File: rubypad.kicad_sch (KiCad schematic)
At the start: 32 parts, among them J1 HRO-TYPE-C, SW1 SW_Push, SW2 RotaryEncoder_Switch, U1 ATmega32U4-A, Y1 16MHz

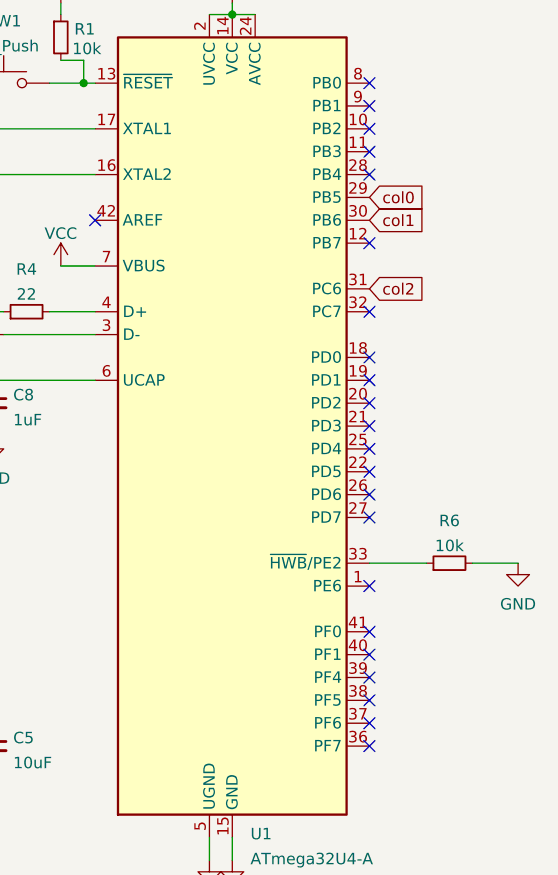
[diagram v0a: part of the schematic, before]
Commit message: changes and complete
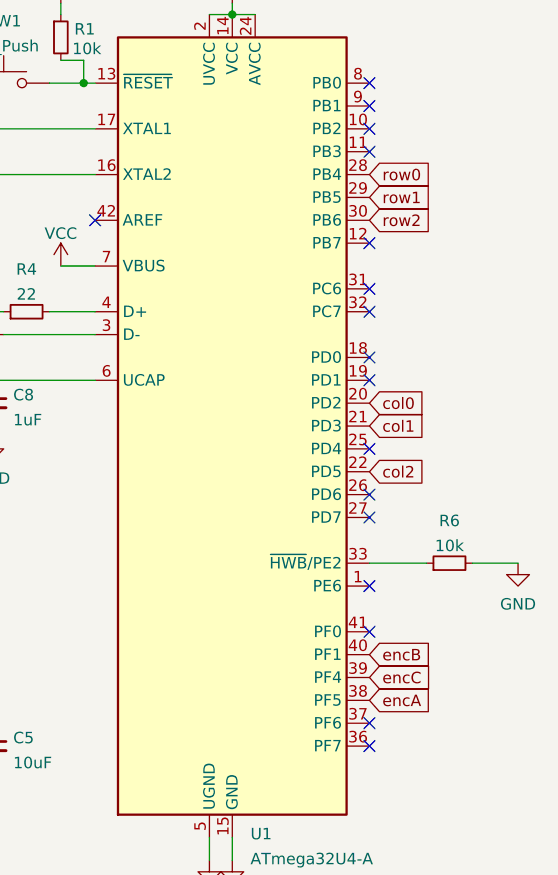
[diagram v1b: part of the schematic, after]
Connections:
- net col0: now also U1.20 (PD2); no longer U1.29 (PB5)
- net col1: now also U1.21 (PD3); no longer U1.30 (PB6)
- net col2: now also U1.22 (PD5); no longer U1.31 (PC6)
- net encA: now also U1.38 (PF5)
- net encB: now also U1.40 (PF1)
- net encC: now also U1.39 (PF4)
- net row0: now also U1.28 (PB4)
- net row1: now also U1.29 (PB5)
- net row2: now also U1.30 (PB6)
- no-connect marks 23 -> 17
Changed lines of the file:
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@@
   (no_connect (at 160.02 74.93))
   (no_connect (at 160.02 72.39))
-  (no_connect (at 160.02 69.85))
   (no_connect (at 160.02 67.31))
-  (no_connect (at 160.02 64.77))
-  (no_connect (at 160.02 95.25))
-  (no_connect (at 160.02 92.71))
-  (no_connect (at 160.02 90.17))
   (no_connect (at 160.02 87.63))
   (no_connect (at 160.02 82.55))
-  (no_connect (at 160.02 62.23))
   (no_connect (at 160.02 59.69))
   (no_connect (at 160.02 57.15))
   (no_connect (at 160.02 52.07))
   (no_connect (at 160.02 44.45))
-  (no_connect (at 160.02 36.83))
   (no_connect (at 160.02 34.29))
   (no_connect (at 160.02 31.75))
   (no_connect (at 160.02 29.21))
   (no_connect (at 160.02 26.67))
+  (no_connect (at 160.02 49.53))
   (wire (pts (xy 73.66 124.46) (xy 73.66 142.24))
     (stroke (width 0) (type default) (color 0 0 0 0))
@@
     )
   )
-  (global_label "col0" (shape input) (at 160.02 39.37 0) (fields_autoplaced)
-    (effects (font (size 1.27 1.27)) (justify left))
-    (property "Intersheet References" "${INTERSHEET_REFS}" (id 0) (at 166.5455 39.2906 0)
+  (global_label "col1" (shape input) (at 160.02 64.77 0) (fields_autoplaced)
+    (effects (font (size 1.27 1.27)) (justify left))
+    (property "Intersheet References" "${INTERSHEET_REFS}" (id 0) (at 166.5455 64.6906 0)
       (effects (font (size 1.27 1.27)) (justify left) hide)
     )
@@
     )
   )
+  (global_label "col0" (shape input) (at 160.02 62.23 0) (fields_autoplaced)
+    (effects (font (size 1.27 1.27)) (justify left))
+    (property "Intersheet References" "${INTERSHEET_REFS}" (id 0) (at 166.5455 62.1506 0)
+      (effects (font (size 1.27 1.27)) (justify left) hide)
+    )
+  )
   (global_label "col2" (shape input) (at 73.66 91.44 90) (fields_autoplaced)
     (effects (font (size 1.27 1.27)) (justify left))
@@
     )
   )
-  (global_label "col1" (shape input) (at 160.02 41.91 0) (fields_autoplaced)
-    (effects (font (size 1.27 1.27)) (justify left))
-    (property "Intersheet References" "${INTERSHEET_REFS}" (id 0) (at 166.5455 41.8306 0)
+  (global_label "encC" (shape input) (at 160.02 92.71 0) (fields_autoplaced)
+    (effects (font (size 1.27 1.27)) (justify left))
+    (property "Intersheet References" "${INTERSHEET_REFS}" (id 0) (at 167.0293 92.7894 0)
       (effects (font (size 1.27 1.27)) (justify left) hide)
     )
@@
     )
   )
+  (global_label "row2" (shape input) (at 160.02 41.91 0) (fields_autoplaced)
+    (effects (font (size 1.27 1.27)) (justify left))
+    (property "Intersheet References" "${INTERSHEET_REFS}" (id 0) (at 166.9083 41.9894 0)
+      (effects (font (size 1.27 1.27)) (justify left) hide)
+    )
+  )
+  (global_label "encB" (shape input) (at 160.02 90.17 0) (fields_autoplaced)
+    (effects (font (size 1.27 1.27)) (justify left))
+    (property "Intersheet References" "${INTERSHEET_REFS}" (id 0) (at 167.0293 90.2494 0)
+      (effects (font (size 1.27 1.27)) (justify left) hide)
+    )
+  )
+  (global_label "col2" (shape input) (at 160.02 69.85 0) (fields_autoplaced)
+    (effects (font (size 1.27 1.27)) (justify left))
+    (property "Intersheet References" "${INTERSHEET_REFS}" (id 0) (at 166.5455 69.7706 0)
+      (effects (font (size 1.27 1.27)) (justify left) hide)
+    )
+  )
   (global_label "D+" (shape input) (at 62.23 49.53 0) (fields_autoplaced)
     (effects (font (size 1.27 1.27)) (justify left))
@@
     )
   )
-  (global_label "col2" (shape input) (at 160.02 49.53 0) (fields_autoplaced)
-    (effects (font (size 1.27 1.27)) (justify left))
-    (property "Intersheet References" "${INTERSHEET_REFS}" (id 0) (at 166.5455 49.4506 0)
-      (effects (font (size 1.27 1.27)) (justify left) hide)
-    )
-  )
   (global_label "D-" (shape input) (at 107.95 54.61 180) (fields_autoplaced)
     (effects (font (size 1.27 1.27)) (justify right))
@@
     )
   )
+  (global_label "row0" (shape input) (at 160.02 36.83 0) (fields_autoplaced)
+    (effects (font (size 1.27 1.27)) (justify left))
+    (property "Intersheet References" "${INTERSHEET_REFS}" (id 0) (at 166.9083 36.9094 0)
+      (effects (font (size 1.27 1.27)) (justify left) hide)
+    )
+  )
   (global_label "encA" (shape input) (at 36.83 101.6 180) (fields_autoplaced)
     (effects (font (size 1.27 1.27)) (justify right))
@@
     )
   )
+  (global_label "encA" (shape input) (at 160.02 95.25 0) (fields_autoplaced)
+    (effects (font (size 1.27 1.27)) (justify left))
+    (property "Intersheet References" "${INTERSHEET_REFS}" (id 0) (at 166.8479 95.3294 0)
+      (effects (font (size 1.27 1.27)) (justify left) hide)
+    )
+  )
   (global_label "encC" (shape input) (at 36.83 104.14 180) (fields_autoplaced)
     (effects (font (size 1.27 1.27)) (justify right))
@@
     )
   )
+  (global_label "row1" (shape input) (at 160.02 39.37 0) (fields_autoplaced)
+    (effects (font (size 1.27 1.27)) (justify left))
+    (property "Intersheet References" "${INTERSHEET_REFS}" (id 0) (at 166.9083 39.4494 0)
+      (effects (font (size 1.27 1.27)) (justify left) hide)
+    )
+  )

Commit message: udpate - going to redo pcb again
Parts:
- Y1: footprint Crystal:Crystal_SMD_3225-4Pin_3.2x2.5mm_HandSoldering -> Crystal:Crystal_SMD_SeikoEpson_TSX3225-4Pin_3.2x2.5mm_HandSoldering
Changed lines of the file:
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@@
     (property "Reference" "Y1" (id 0) (at 114.3 33.02 90))
     (property "Value" "16MHz" (id 1) (at 114.3 35.56 90))
-    (property "Footprint" "Crystal:Crystal_SMD_3225-4Pin_3.2x2.5mm_HandSoldering" (id 2) (at 106.68 34.29 0)
+    (property "Footprint" "Crystal:Crystal_SMD_SeikoEpson_TSX3225-4Pin_3.2x2.5mm_HandSoldering" (id 2) (at 106.68 34.29 0)
       (effects (font (size 1.27 1.27)) hide)
     )
@@
     )
     (path "/a3f5d478-605e-4e12-a2a8-da8d8a4a13a3"
-      (reference "Y1") (unit 1) (value "16MHz") (footprint "Crystal:Crystal_SMD_3225-4Pin_3.2x2.5mm_HandSoldering")
-    )
-  )
+      (reference "Y1") (unit 1) (value "16MHz") (footprint "Crystal:Crystal_SMD_SeikoEpson_TSX3225-4Pin_3.2x2.5mm_HandSoldering")
+    )
+  )

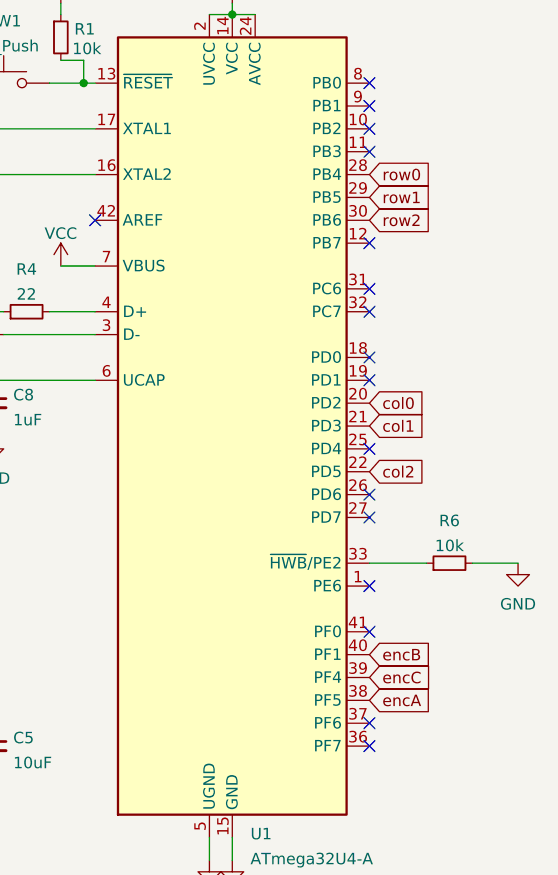
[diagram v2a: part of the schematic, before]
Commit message: udpate
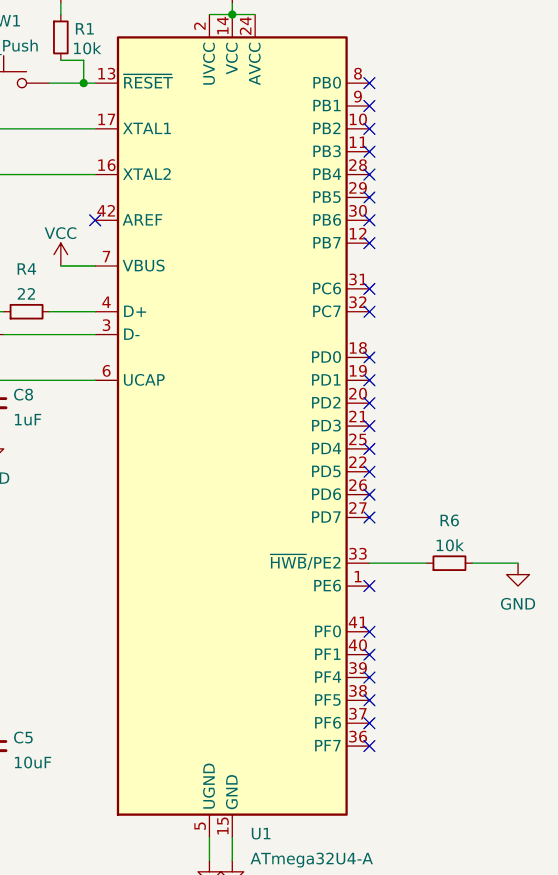
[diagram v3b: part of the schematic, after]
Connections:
- net col0: no longer U1.20 (PD2)
- net col1: no longer U1.21 (PD3)
- net col2: no longer U1.22 (PD5)
- net encA: no longer U1.38 (PF5)
- net encB: no longer U1.40 (PF1)
- net encC: no longer U1.39 (PF4)
- net row0: no longer U1.28 (PB4)
- net row1: no longer U1.29 (PB5)
- net row2: no longer U1.30 (PB6)
- no-connect marks 17 -> 26
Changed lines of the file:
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@@
   (no_connect (at 160.02 26.67))
   (no_connect (at 160.02 49.53))
+  (no_connect (at 160.02 95.25))
+  (no_connect (at 160.02 92.71))
+  (no_connect (at 160.02 90.17))
+  (no_connect (at 160.02 39.37))
+  (no_connect (at 160.02 41.91))
+  (no_connect (at 160.02 64.77))
+  (no_connect (at 160.02 62.23))
+  (no_connect (at 160.02 69.85))
+  (no_connect (at 160.02 36.83))
   (wire (pts (xy 73.66 124.46) (xy 73.66 142.24))
     (stroke (width 0) (type default) (color 0 0 0 0))
@@
     (property "Intersheet References" "${INTERSHEET_REFS}" (id 0) (at 24.8617 152.3206 0)
       (effects (font (size 1.27 1.27)) (justify right) hide)
-    )
-  )
-  (global_label "col1" (shape input) (at 160.02 64.77 0) (fields_autoplaced)
-    (effects (font (size 1.27 1.27)) (justify left))
-    (property "Intersheet References" "${INTERSHEET_REFS}" (id 0) (at 166.5455 64.6906 0)
-      (effects (font (size 1.27 1.27)) (justify left) hide)
     )
   )
@@
     )
   )
-  (global_label "col0" (shape input) (at 160.02 62.23 0) (fields_autoplaced)
-    (effects (font (size 1.27 1.27)) (justify left))
-    (property "Intersheet References" "${INTERSHEET_REFS}" (id 0) (at 166.5455 62.1506 0)
-      (effects (font (size 1.27 1.27)) (justify left) hide)
-    )
-  )
   (global_label "col2" (shape input) (at 73.66 91.44 90) (fields_autoplaced)
     (effects (font (size 1.27 1.27)) (justify left))
@@
     )
   )
-  (global_label "encC" (shape input) (at 160.02 92.71 0) (fields_autoplaced)
-    (effects (font (size 1.27 1.27)) (justify left))
-    (property "Intersheet References" "${INTERSHEET_REFS}" (id 0) (at 167.0293 92.7894 0)
-      (effects (font (size 1.27 1.27)) (justify left) hide)
-    )
-  )
   (global_label "row1" (shape input) (at 31.75 134.62 180) (fields_autoplaced)
     (effects (font (size 1.27 1.27)) (justify right))
     (property "Intersheet References" "${INTERSHEET_REFS}" (id 0) (at 24.8617 134.5406 0)
       (effects (font (size 1.27 1.27)) (justify right) hide)
-    )
-  )
-  (global_label "row2" (shape input) (at 160.02 41.91 0) (fields_autoplaced)
-    (effects (font (size 1.27 1.27)) (justify left))
-    (property "Intersheet References" "${INTERSHEET_REFS}" (id 0) (at 166.9083 41.9894 0)
-      (effects (font (size 1.27 1.27)) (justify left) hide)
-    )
-  )
-  (global_label "encB" (shape input) (at 160.02 90.17 0) (fields_autoplaced)
-    (effects (font (size 1.27 1.27)) (justify left))
-    (property "Intersheet References" "${INTERSHEET_REFS}" (id 0) (at 167.0293 90.2494 0)
-      (effects (font (size 1.27 1.27)) (justify left) hide)
-    )
-  )
-  (global_label "col2" (shape input) (at 160.02 69.85 0) (fields_autoplaced)
-    (effects (font (size 1.27 1.27)) (justify left))
-    (property "Intersheet References" "${INTERSHEET_REFS}" (id 0) (at 166.5455 69.7706 0)
-      (effects (font (size 1.27 1.27)) (justify left) hide)
     )
   )
@@
     )
   )
-  (global_label "row0" (shape input) (at 160.02 36.83 0) (fields_autoplaced)
-    (effects (font (size 1.27 1.27)) (justify left))
-    (property "Intersheet References" "${INTERSHEET_REFS}" (id 0) (at 166.9083 36.9094 0)
-      (effects (font (size 1.27 1.27)) (justify left) hide)
-    )
-  )
   (global_label "encA" (shape input) (at 36.83 101.6 180) (fields_autoplaced)
     (effects (font (size 1.27 1.27)) (justify right))
@@
     )
   )
-  (global_label "encA" (shape input) (at 160.02 95.25 0) (fields_autoplaced)
-    (effects (font (size 1.27 1.27)) (justify left))
-    (property "Intersheet References" "${INTERSHEET_REFS}" (id 0) (at 166.8479 95.3294 0)
-      (effects (font (size 1.27 1.27)) (justify left) hide)
-    )
-  )
   (global_label "encC" (shape input) (at 36.83 104.14 180) (fields_autoplaced)
     (effects (font (size 1.27 1.27)) (justify right))
@@
     )
   )
-  (global_label "row1" (shape input) (at 160.02 39.37 0) (fields_autoplaced)
-    (effects (font (size 1.27 1.27)) (justify left))
-    (property "Intersheet References" "${INTERSHEET_REFS}" (id 0) (at 166.9083 39.4494 0)
-      (effects (font (size 1.27 1.27)) (justify left) hide)
-    )
-  )
